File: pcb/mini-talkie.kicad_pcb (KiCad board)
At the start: 2 copper layers, 47 parts, among them J1 SWD, J2 USB_C_Receptacle_USB2.0_16P, J3 BATT, J4 SPEAKER, Q1 AO3401A, SW1 SW_SP3T, SW2 SW_SPDT, SW3 SW_SPST, U1 STM32H503CBTx, U2 Wio-SX1262, U3 PAM8302AAS, U4 MCP73831-2-OT, U5 RT9080

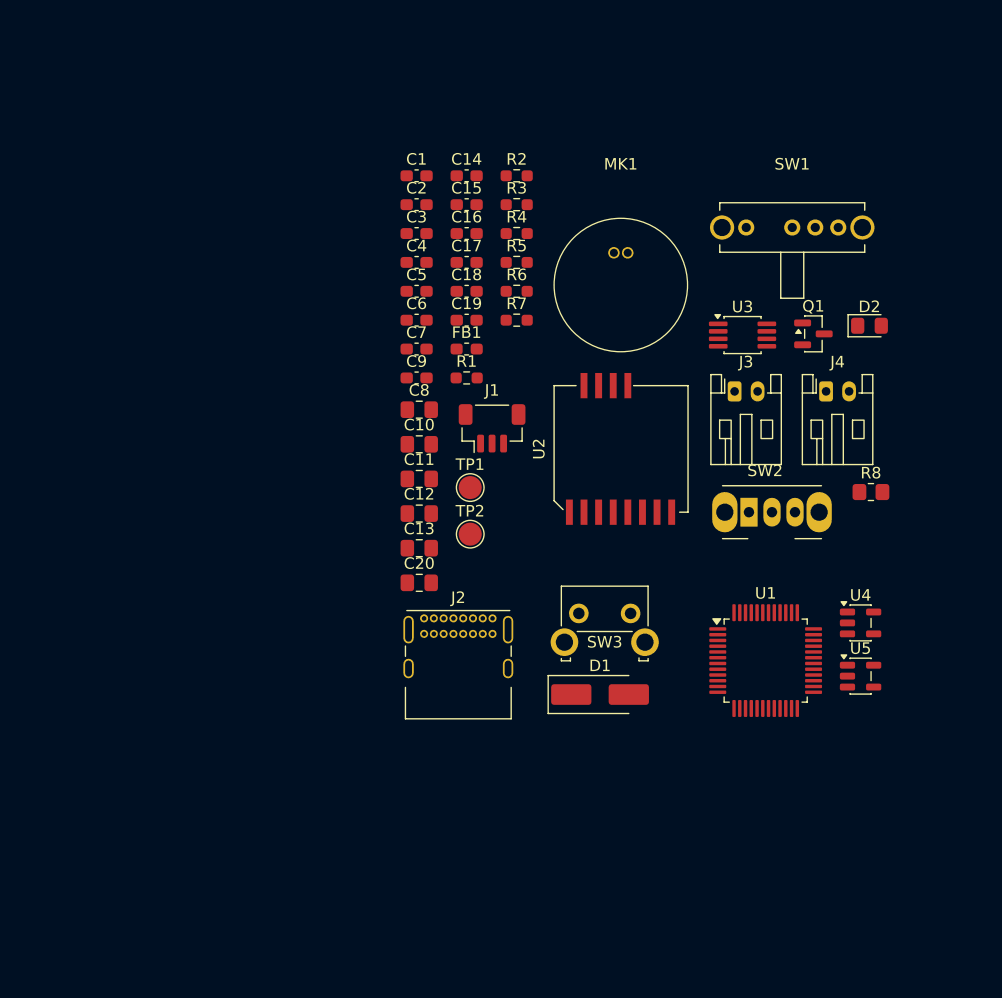
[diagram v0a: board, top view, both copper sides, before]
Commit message: get started with layout
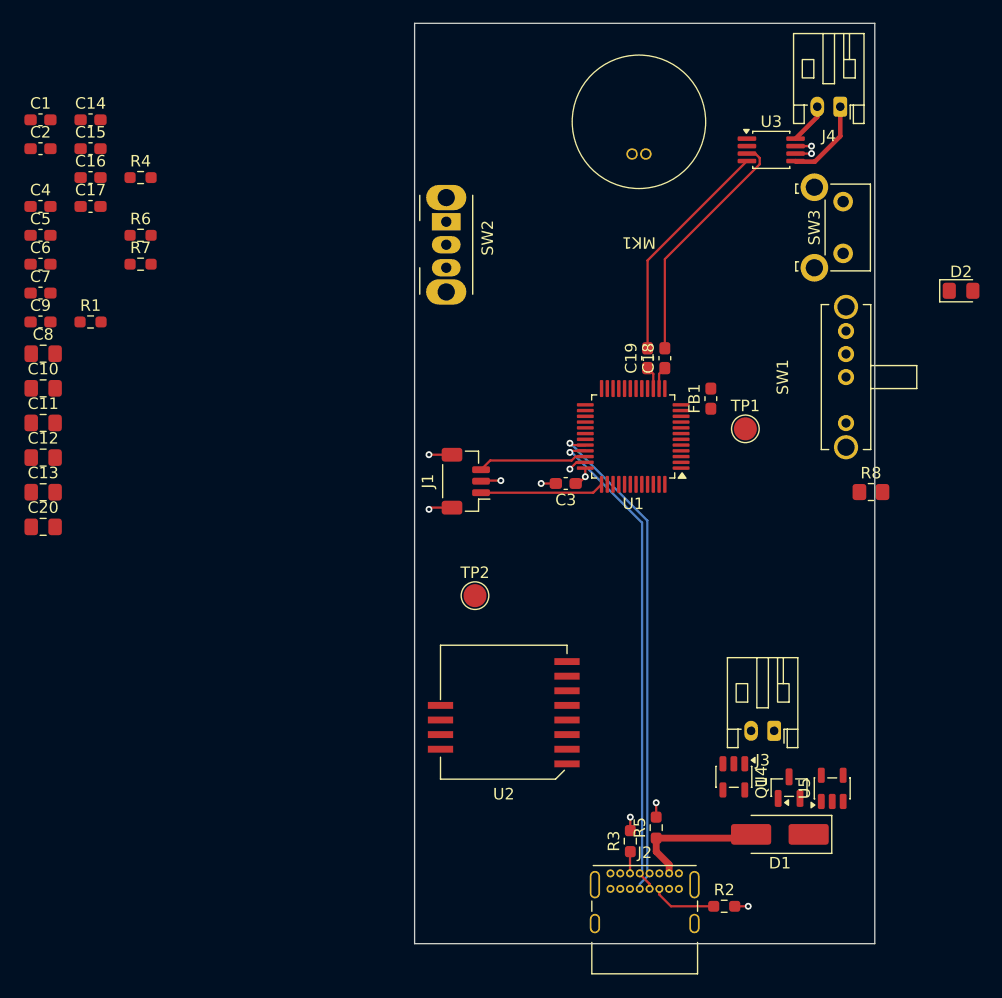
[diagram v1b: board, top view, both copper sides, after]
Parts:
- moved R2 66.0 mm to (155.4, 141.8)
- moved R3 56.2 mm to (147.2, 136.1), turned to 90 degrees
- moved R5 50.6 mm to (149.5, 134.9), turned to 90 degrees
- moved SW3 42.5 mm to (165.8, 80.5), turned to -90 degrees
- moved Q1 39.5 mm to (161.1, 131.4), turned to 90 degrees
- moved SW2 36.5 mm to (131.2, 82.2), turned to -90 degrees
- moved C16 33.1 mm to (100.3, 78.4)
- moved C6 33.1 mm to (96.0, 85.9)
- moved C9 33.1 mm to (96.0, 91.0)
- moved R1 33.1 mm to (100.3, 91.0)
- moved C1 33.1 mm to (96.0, 73.4)
- moved C14 33.1 mm to (100.3, 73.4)
- moved C15 33.1 mm to (100.3, 75.9)
- moved C17 33.1 mm to (100.3, 80.9)
- moved C2 33.1 mm to (96.0, 75.9)
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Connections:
- SW1 pad 1: unconnected-(SW1-Pad1) -> /MODE_VA
- SW1 pad 2: unconnected-(SW1-Pad2) -> /MODE_PTT
- SW1 pad 3: unconnected-(SW1-Pad3) -> /MODE_C
- SW1 pad 4: unconnected-(SW1-Pad4) -> /MODE_M
- SW3 pad 1: unconnected-(SW3-A-Pad1) -> /PTT_IN
- SW3 pad 2: unconnected-(SW3-B-Pad2) -> /PTT_OUT
- U1 pad 25: unconnected-(U1-PB12-Pad25) -> /MODE_C
- U1 pad 26: unconnected-(U1-PB13-Pad26) -> /MODE_VA
- U1 pad 27: unconnected-(U1-PB14-Pad27) -> /MODE_PTT
- U1 pad 28: unconnected-(U1-PB15-Pad28) -> /MODE_M
- U1 pad 29: unconnected-(U1-PA8-Pad29) -> /PTT_IN
- U1 pad 30: unconnected-(U1-PA9-Pad30) -> /PTT_OUT
- U1 pad 32: unconnected-(U1-PA11-Pad32) -> /USB_D-
- U1 pad 33: unconnected-(U1-PA12-Pad33) -> /USB_D+
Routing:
- net /USB_D-: track 0.00 -> 43.4 mm, vias 0 -> 1
- net /USB_D+: track 0.00 -> 42.5 mm, vias 0 -> 1
- net Net-(U3-IN+): track 0.00 -> 21.2 mm
- net VBUS: track 0.00 -> 20.1 mm
- net Net-(U3-IN-): track 0.00 -> 19.9 mm
- net GND: track 0.00 -> 13.7 mm, vias 0 -> 9
- net /SWCLK: track 0.00 -> 10.8 mm
- net /SWDIO: track 0.00 -> 9.53 mm
- net Net-(J4-Pin_1): track 0.00 -> 7.39 mm
- net Net-(J2-CC2): track 0.00 -> 5.64 mm
- net Net-(J4-Pin_2): track 0.00 -> 3.56 mm
- net +3V3: track 0.00 -> 3.22 mm, vias 0 -> 2
- net /IN-: track 0.00 -> 1.98 mm
- net /IN+: track 0.00 -> 1.98 mm
- net Net-(J2-CC1): track 0.00 -> 1.90 mm
- added copper zone on In2.Cu, net +3V3
- added copper zone on In1.Cu, net GND
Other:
- board outline added: 40 x 80 mm
- copper layers 2 -> 4
